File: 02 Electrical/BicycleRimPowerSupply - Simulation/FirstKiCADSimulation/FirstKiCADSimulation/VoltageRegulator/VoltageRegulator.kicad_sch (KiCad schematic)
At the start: 3 parts, among them U1 LM1117-5.0

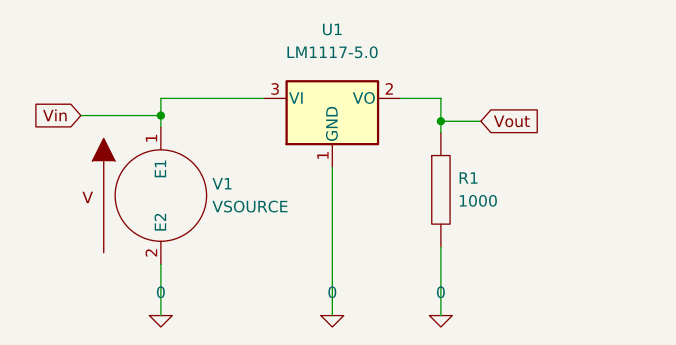
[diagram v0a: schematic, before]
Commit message: PCB design
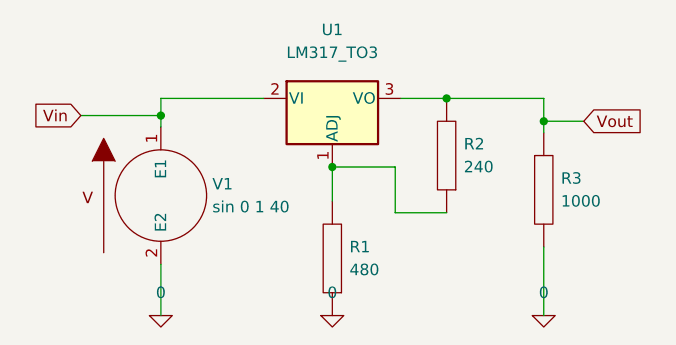
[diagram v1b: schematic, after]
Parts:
- removed U1: LM1117-5.0, symbol Regulator_Linear:LM1117-5.0
- added R1: 480, symbol pspice:R
- added R2: 240, symbol pspice:R
- added U1: LM317_TO3, Package_TO_SOT_THT:TO-3, symbol Regulator_Linear:LM317_TO3
- V1: value VSOURCE -> sin 0 1 40; Spice_Model sin(6 1 100) -> sin(0 1)
- renumbered R1 to R3
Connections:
- net 0: now also R1.1
- net Vin: now also U1.2 (VI)
- net Vout: now also R2.2, U1.3 (VO)
- new net: R1.2, R2.1, U1.1 (ADJ)
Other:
- moved on the sheet: R3
